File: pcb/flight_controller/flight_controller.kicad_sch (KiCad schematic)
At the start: 23 parts, among them J1 USB-C Connector, U1 ICM-42688-P, U2 STM32F405RGT6, U3 XC6219B332MR

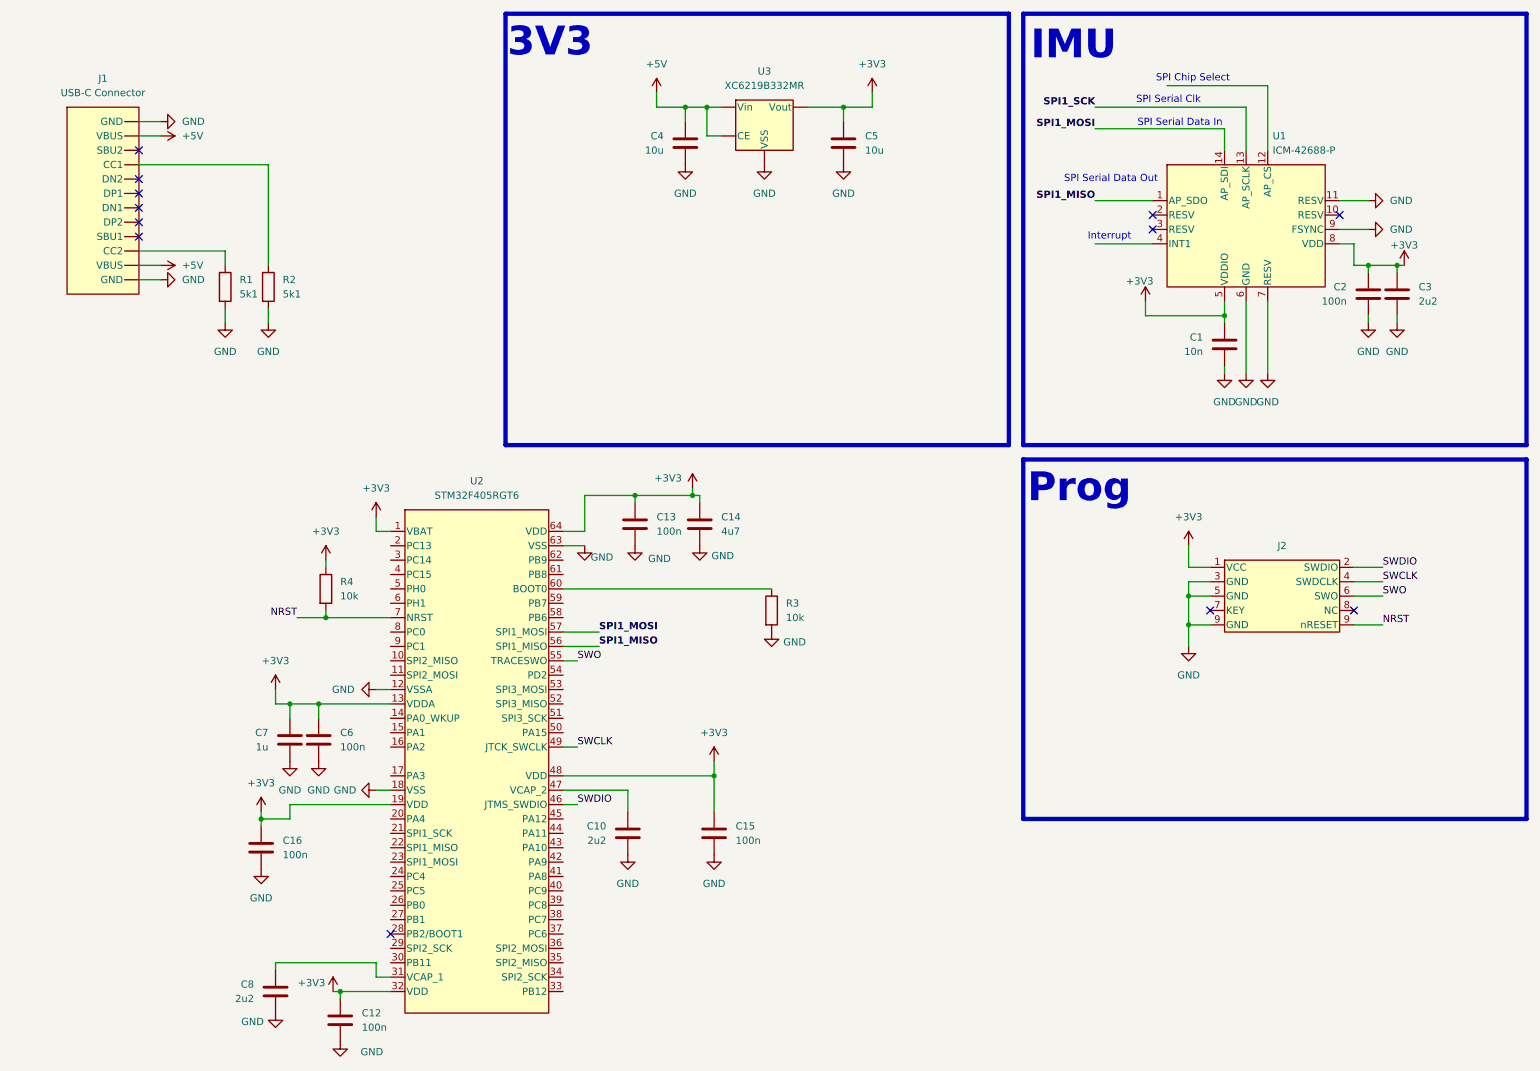
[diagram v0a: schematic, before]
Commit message: initial implementation of crystal
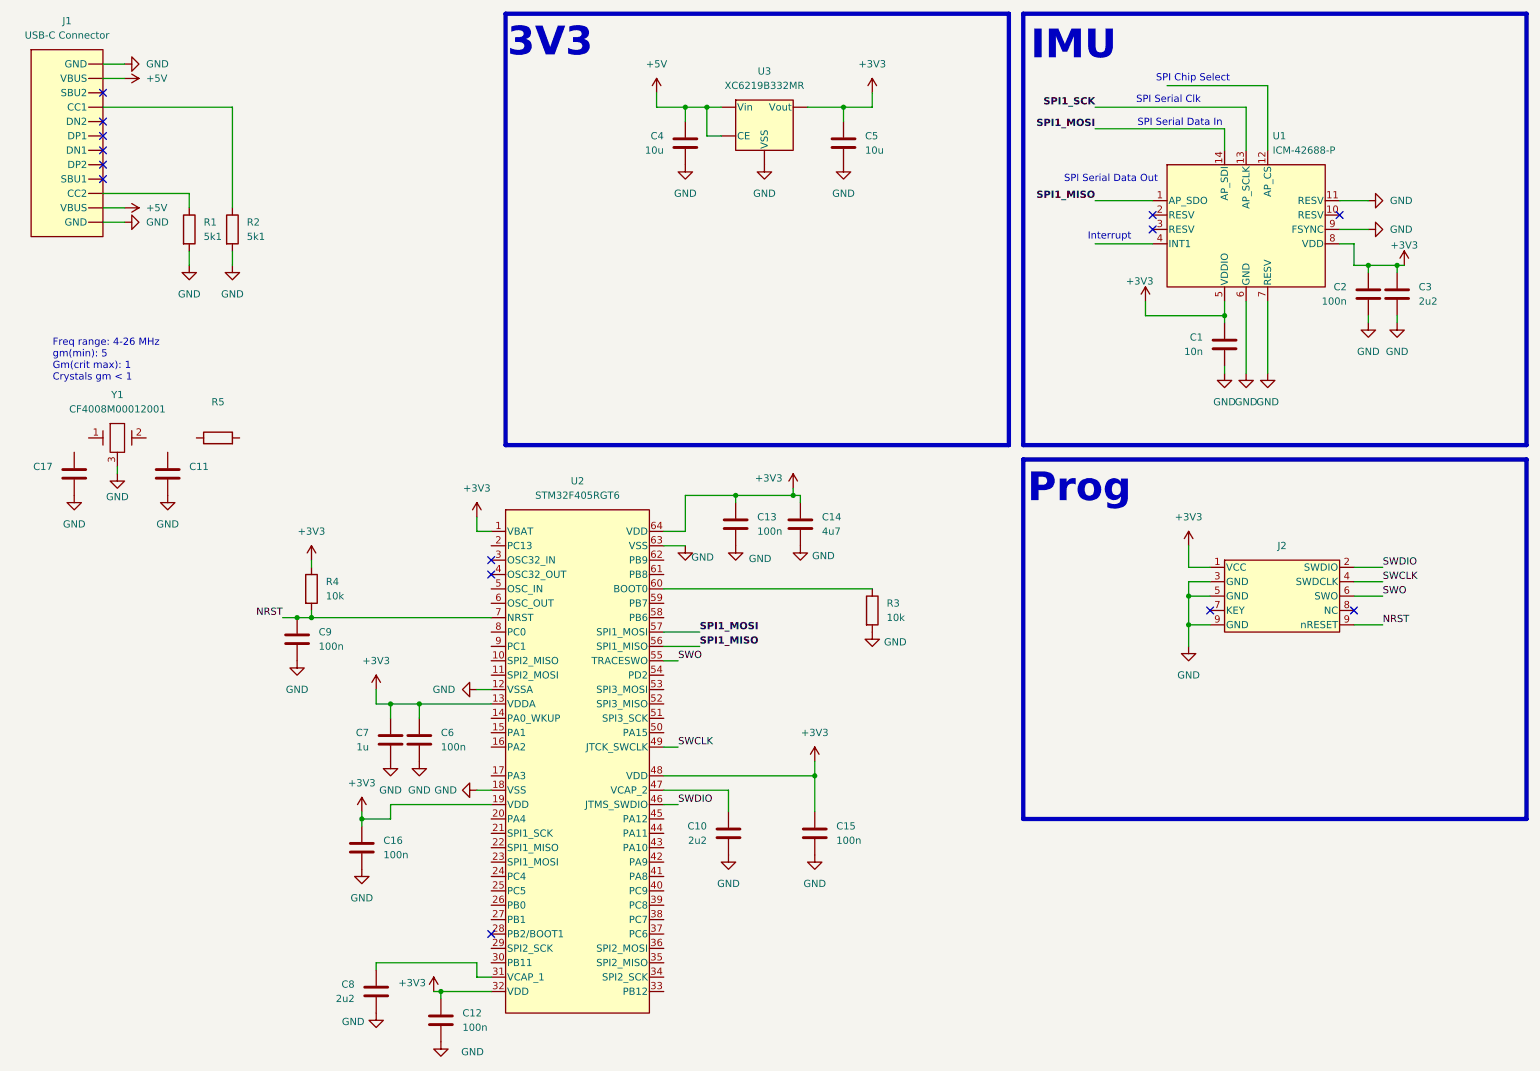
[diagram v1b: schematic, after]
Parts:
- added C11, C17: (no value), symbol Device:C
- added C9: 100n, symbol Device:C
- added R5: (no value), symbol Device:R
- added Y1: CF4008M00012001, symbol symbols_local:CF4008M00012001
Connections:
- net GND: now also C11.1, C17.1, C9.1, Y1.3 (GND)
- net NRST: now also C9.2
- no-connect marks 12 -> 14
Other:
- note added: "Freq range: 4-26 MHz gm(min): 5 Gm(crit max): 1 Crystals gm < 1"
- moved on the sheet: C10, C12, C13, C14, C15, C16, C6, C7, C8, J1, R1, R2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
